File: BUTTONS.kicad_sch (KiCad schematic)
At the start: 11 parts, among them J4 Conn_01x10_Pin, U1 ITR1201SR10AR, U2 ITR1201SR10AR, U3 ITR1201SR10AR, U4 ITR1201SR10AR

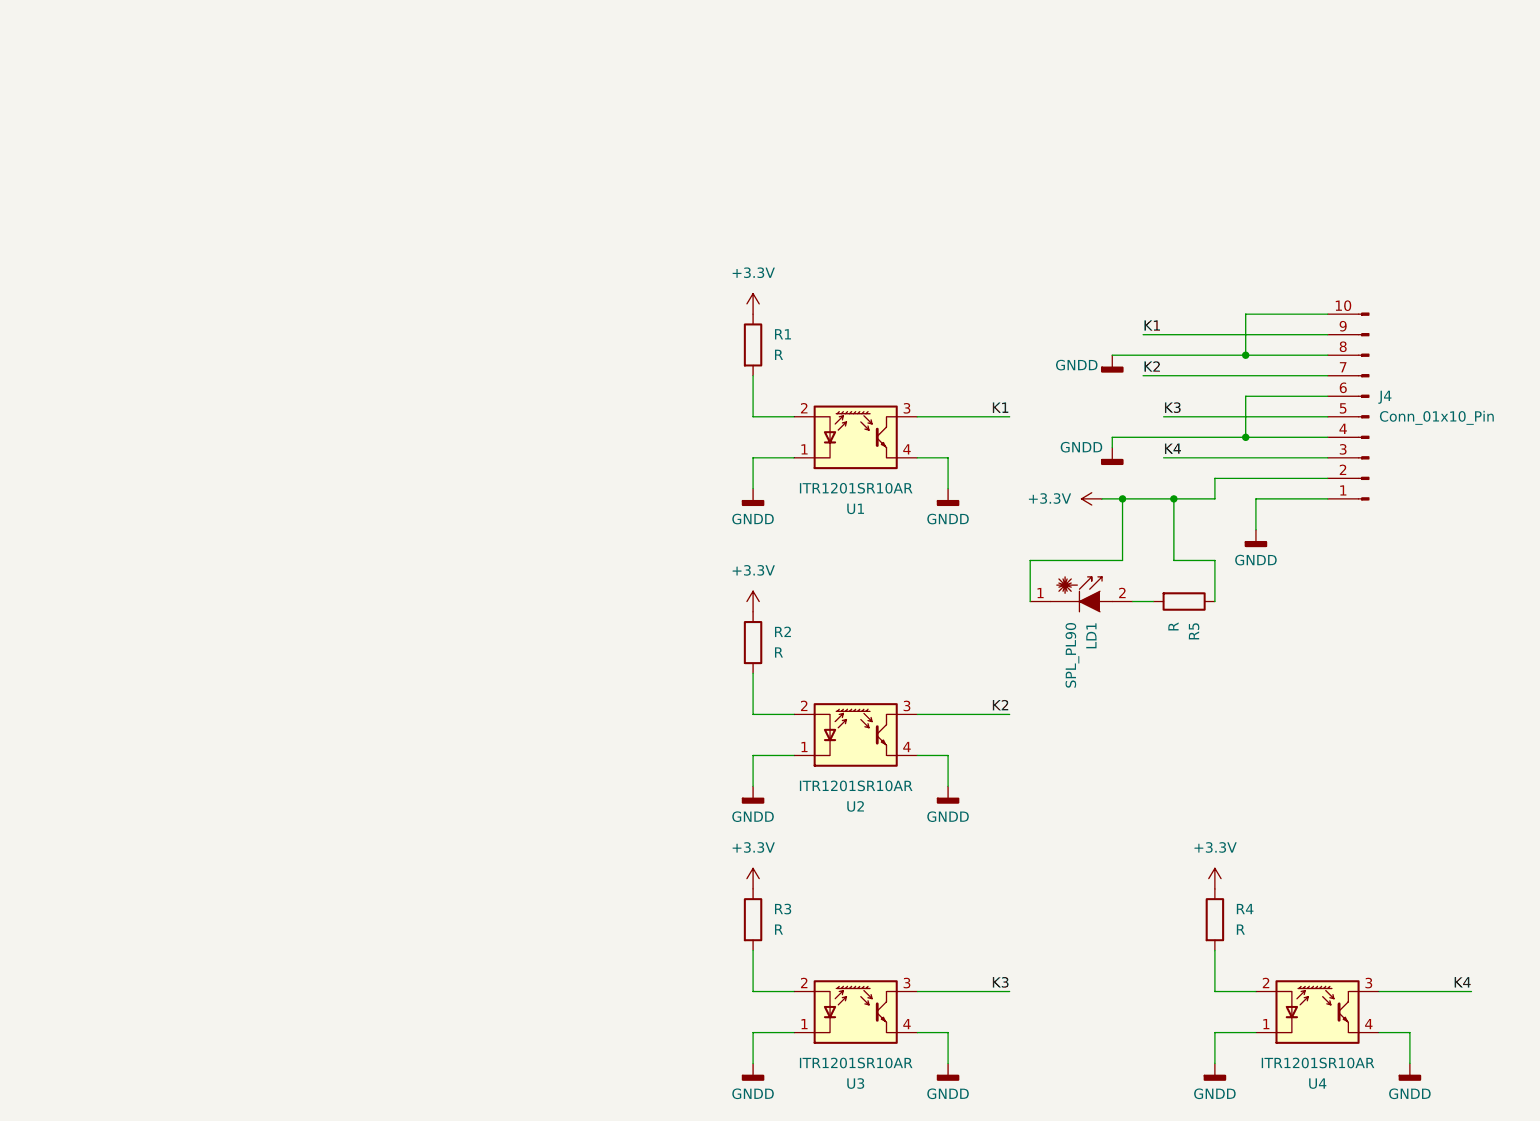
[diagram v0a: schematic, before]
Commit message: Add files via upload
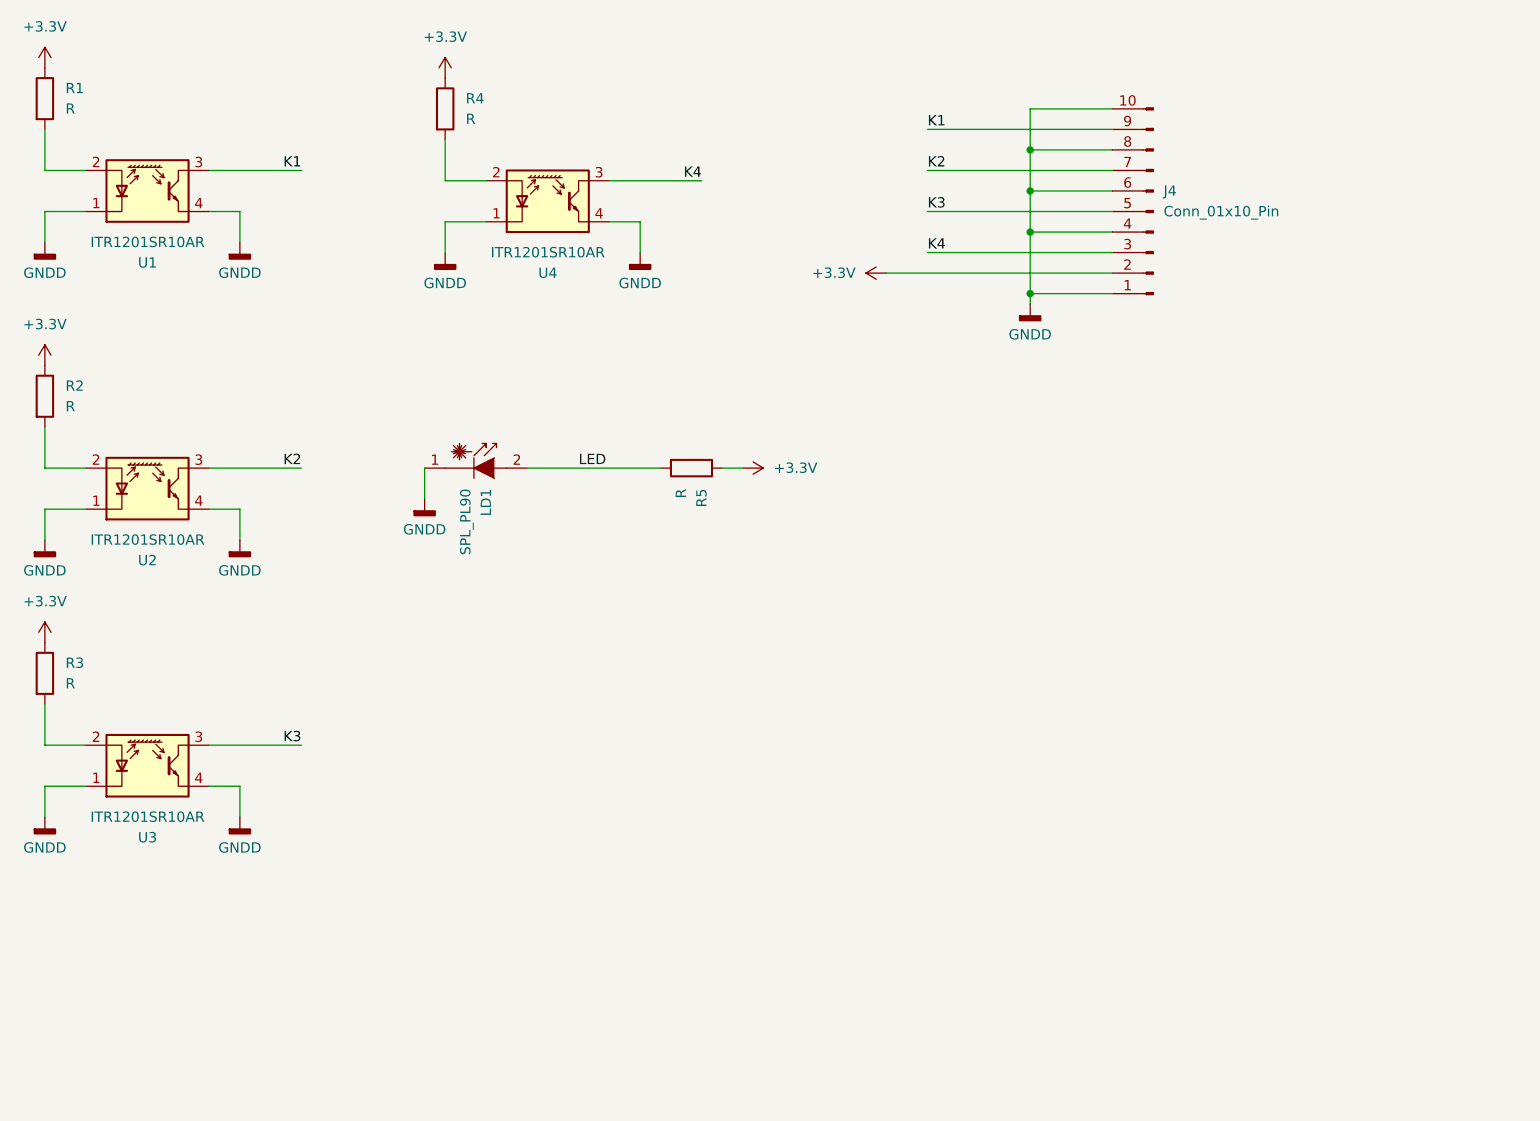
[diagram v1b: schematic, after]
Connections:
- net +3.3V: no longer LD1.1 (C)
- net GNDD: now also LD1.1 (C)
- net LED: now reaches LD1.2 (A), R5.2
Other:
- moved on the sheet: J4, LD1, R1, R2, R3, R4, R5, U1, U2, U3, U4
